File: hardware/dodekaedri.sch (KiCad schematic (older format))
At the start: 16 parts

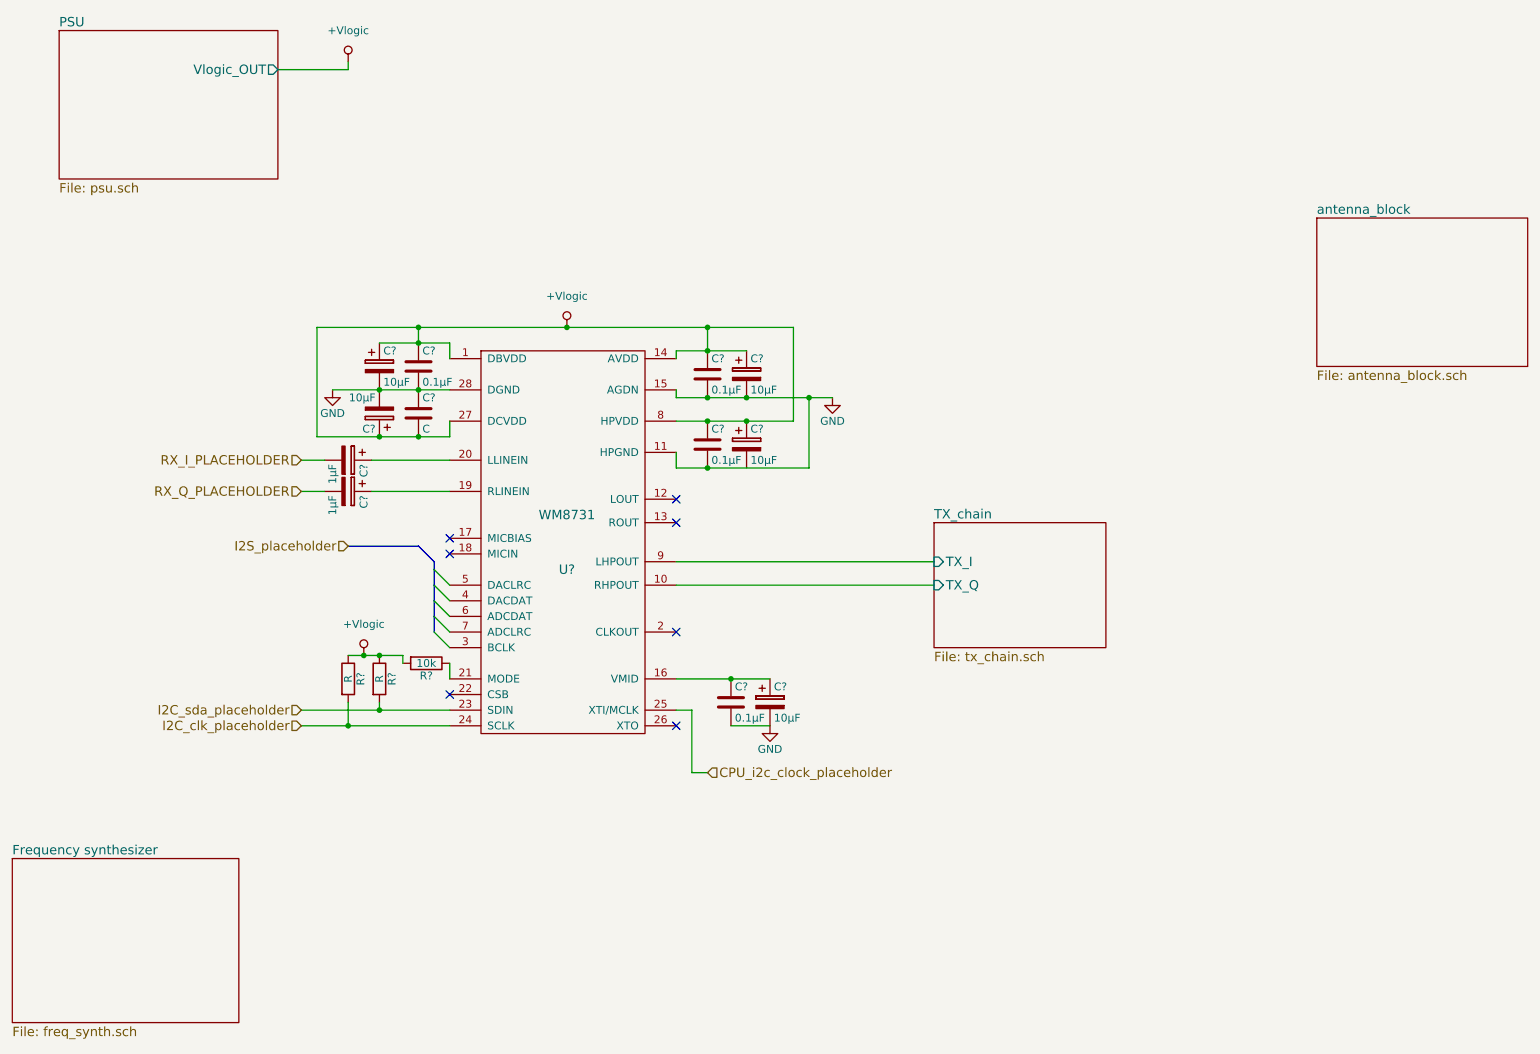
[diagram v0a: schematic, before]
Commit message: honed multiple schematics
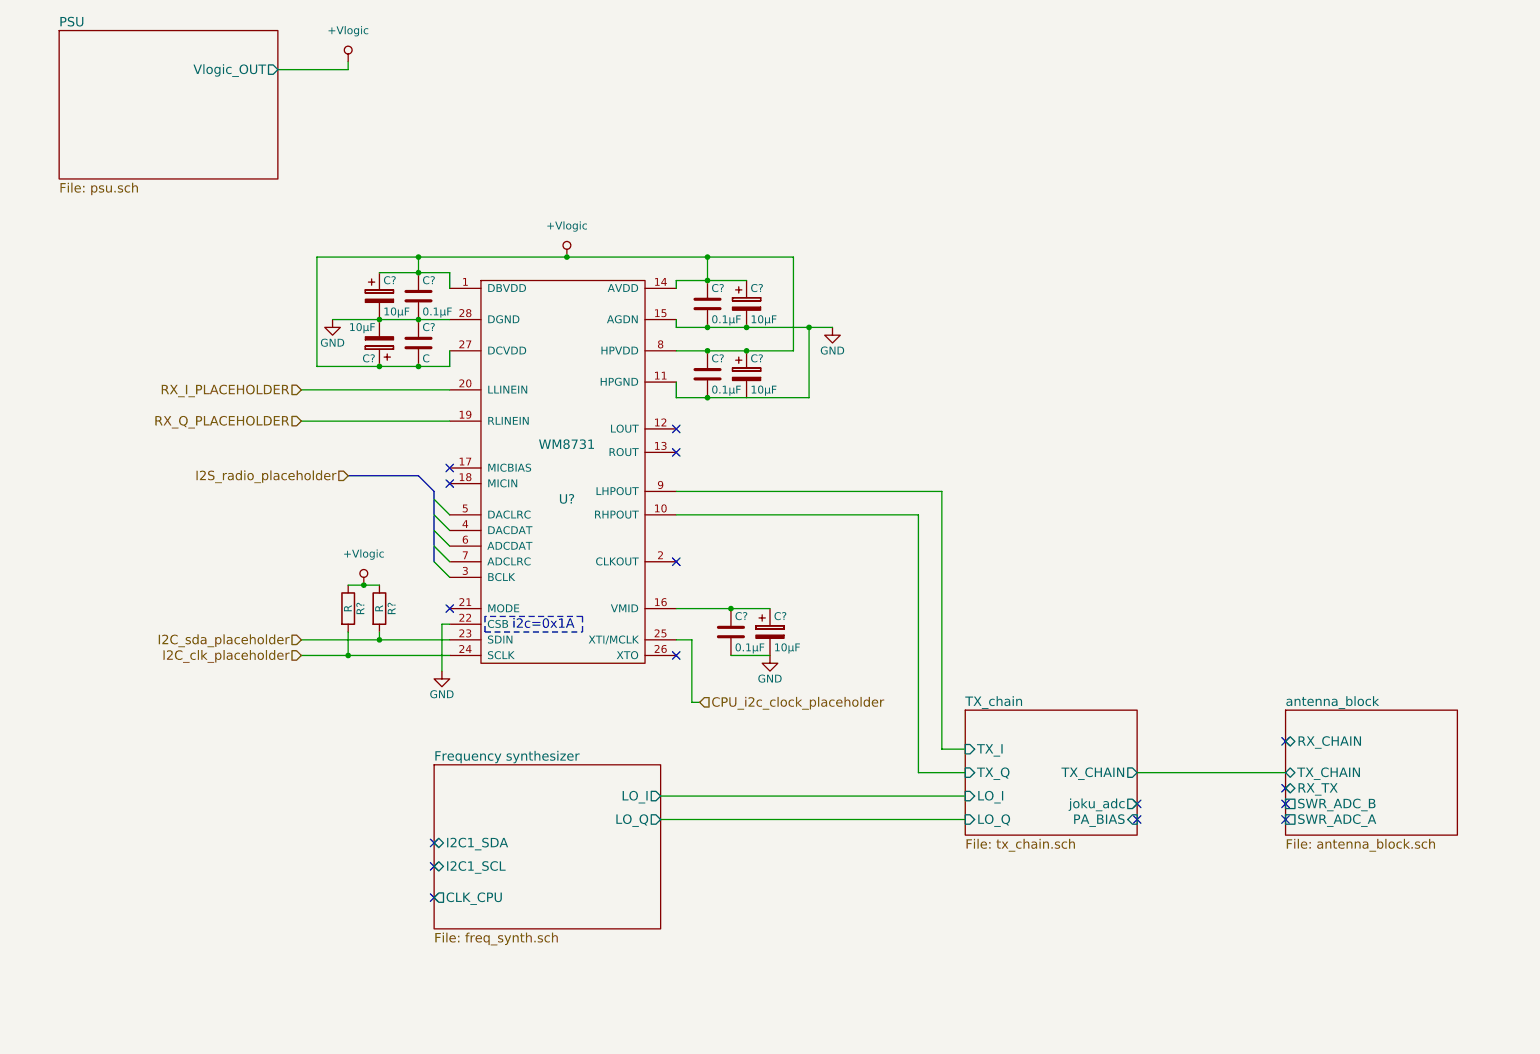
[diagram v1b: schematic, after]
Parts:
- removed C? (x2): 1µF, symbol CP
- removed R?: 10k, symbol R
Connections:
- net GND: now also U?.22 (CSB)
- net RX_I_PLACEHOLDER: now also U?.20 (LLINEIN)
- net RX_Q_PLACEHOLDER: now also U?.19 (RLINEIN)
- no-connect marks 7 -> 16
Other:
- note added: "i2c=0x1A"
- moved on the sheet: C?, R?, U?
